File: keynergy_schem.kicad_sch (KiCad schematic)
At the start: 28 parts, among them J1 Conn_01x04_Pin, J2 Conn_01x04_Pin, J3 Conn_01x02_Pin, J4 Conn_01x04_Pin, J5 Conn_01x04_Pin, J6 Conn_01x04_Pin, J8 Conn_01x04_Pin

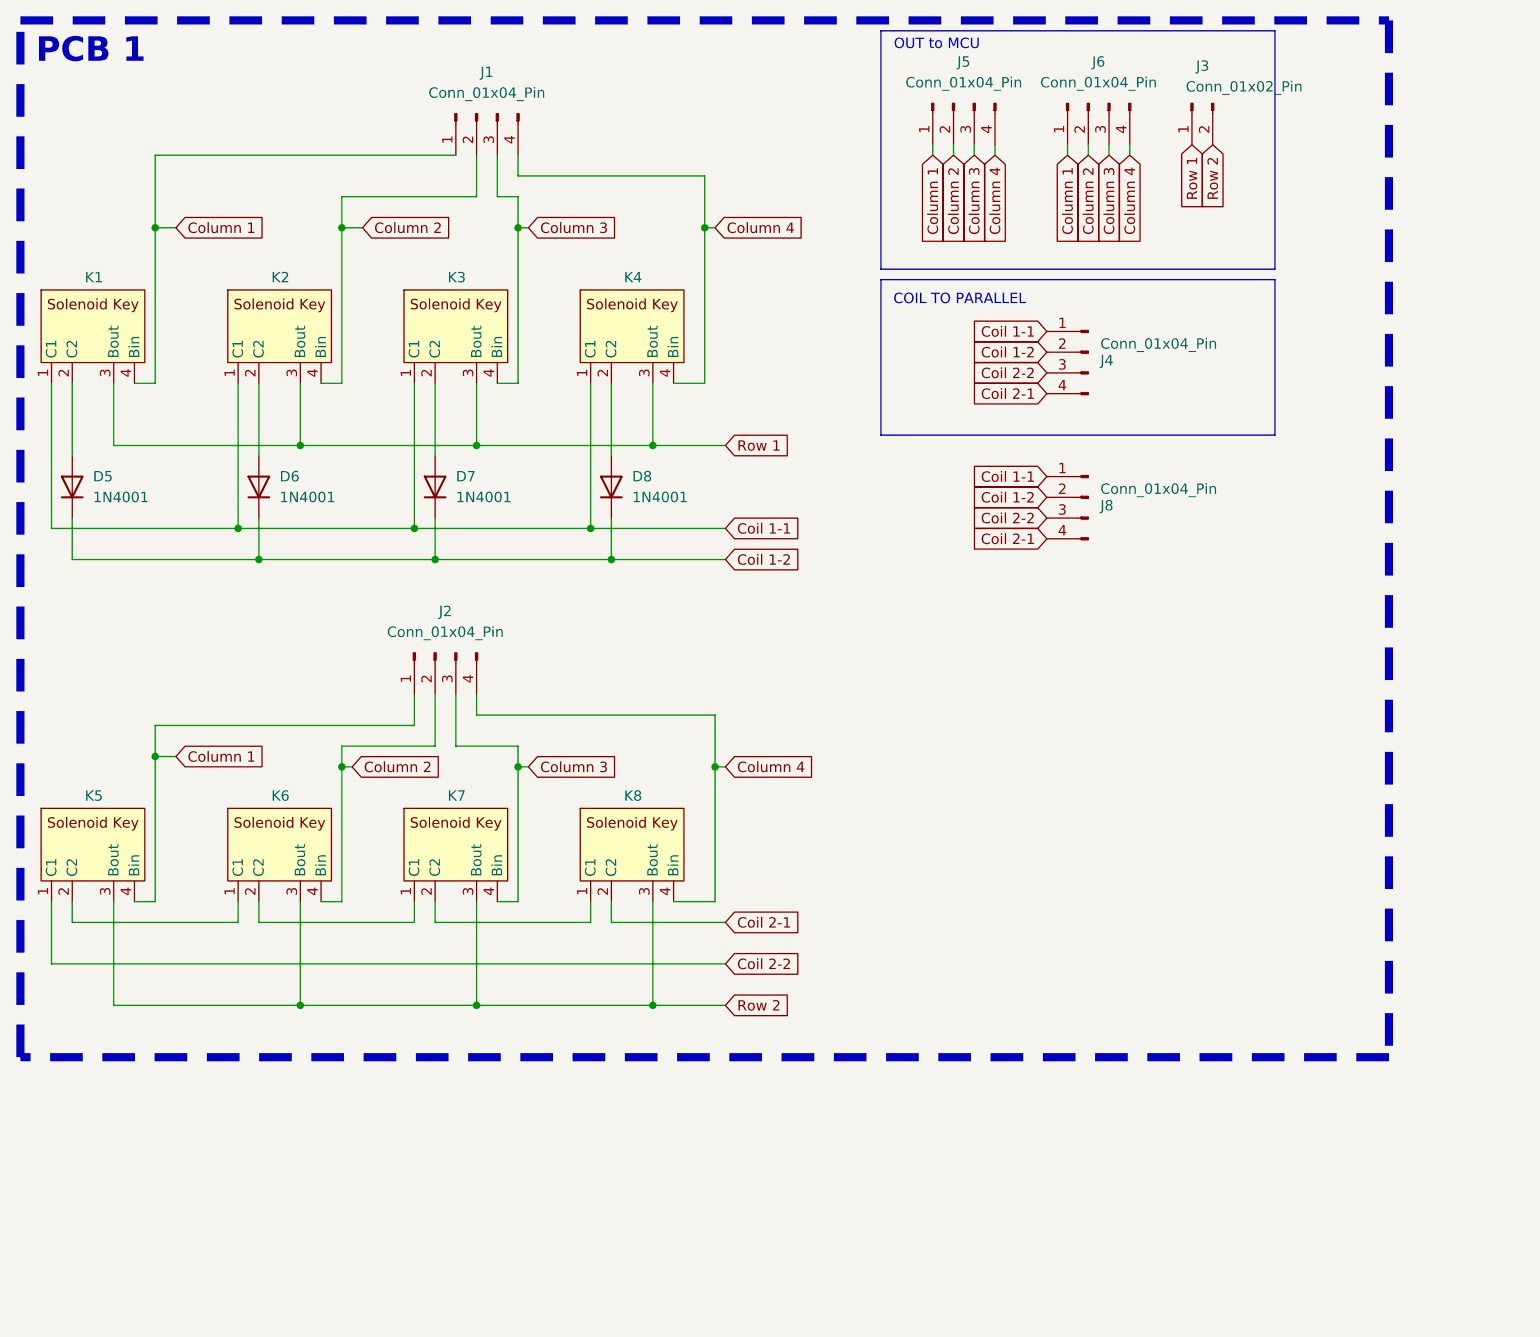
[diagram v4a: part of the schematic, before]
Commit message: new
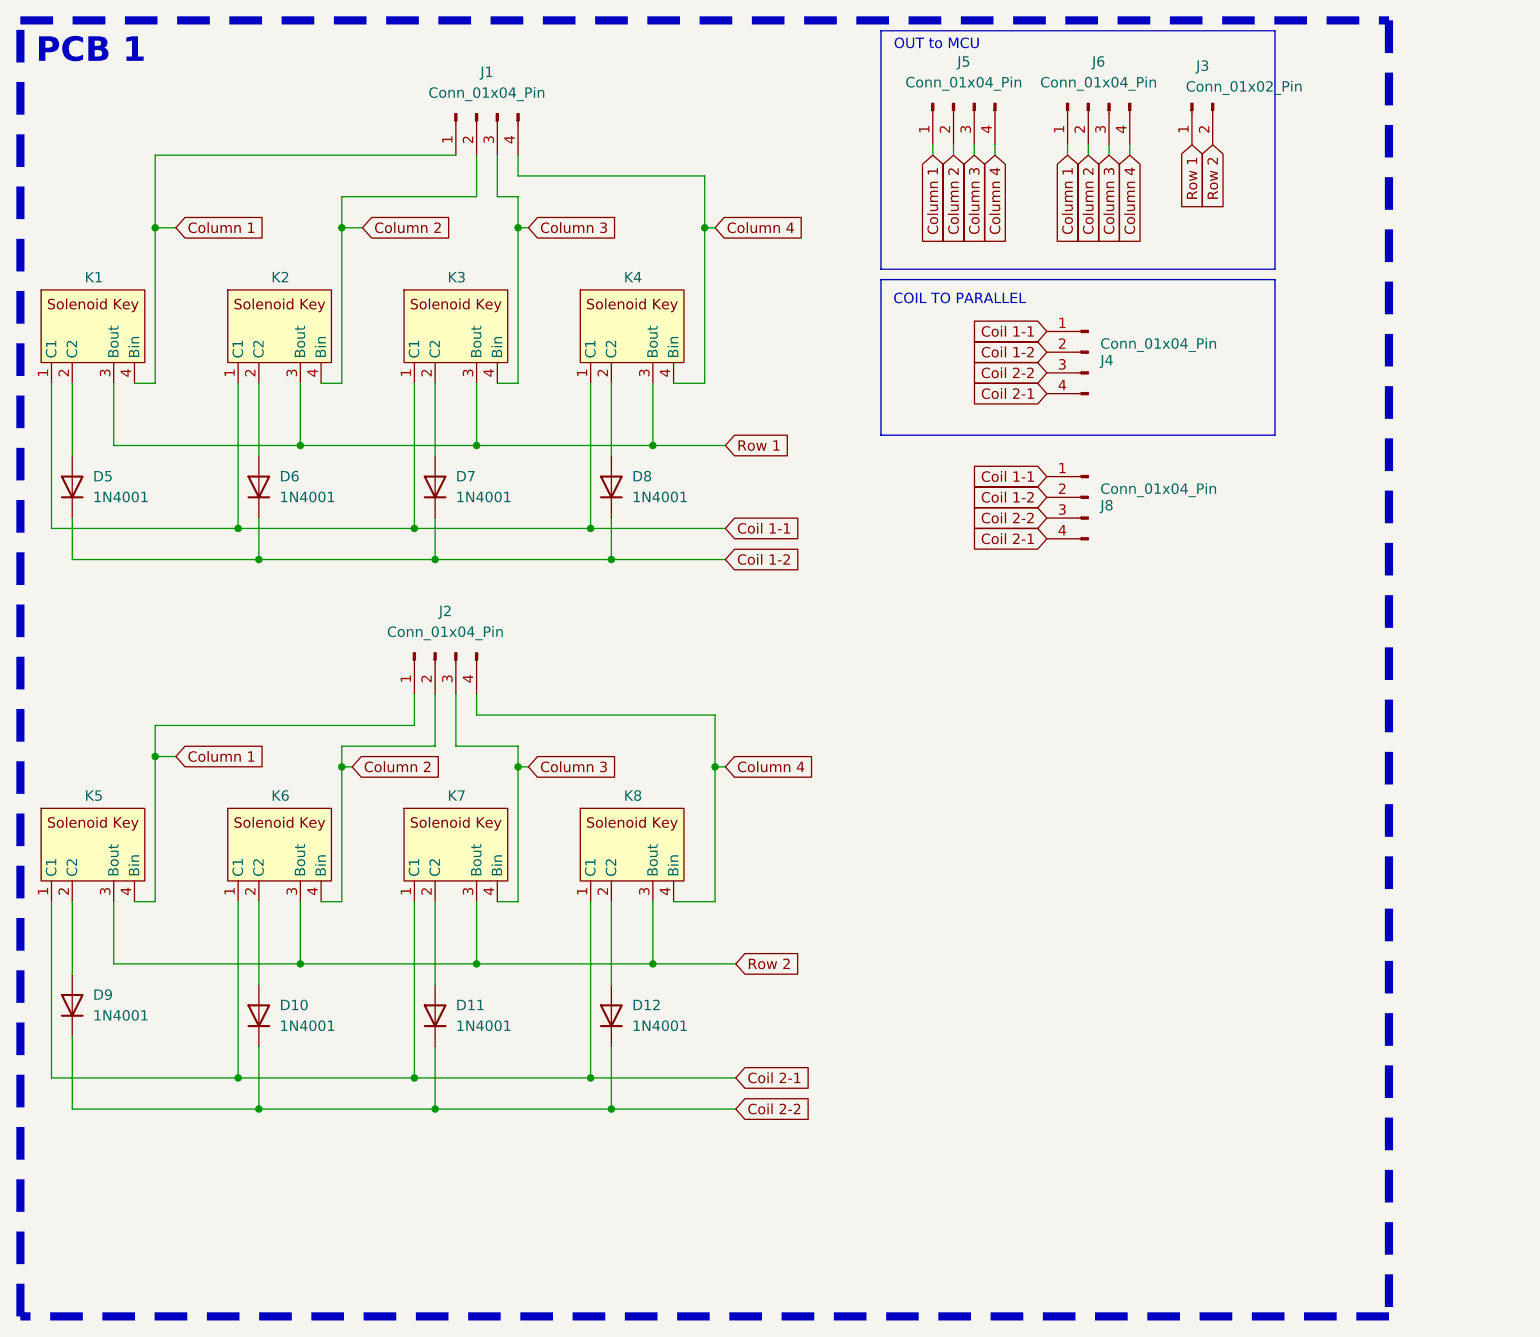
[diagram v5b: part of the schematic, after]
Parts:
- added D10, D11, D12, D9: 1N4001, Diode_THT:D_DO-34_SOD68_P7.62mm_Horizontal, symbol Device:D
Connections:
- net Coil 2-1: now also K5.1 (C1), K6.1 (C1), K7.1 (C1), K8.1 (C1); no longer K8.2 (C2)
- net Coil 2-2: now also D10.1 (K), D11.1 (K), D12.1 (K), D9.1 (K); no longer K5.1 (C1)
- net at K6.2 (C2): now also D10.2 (A); no longer K7.1 (C1)
- net at K7.2 (C2): now also D11.2 (A); no longer K8.1 (C1)
- net at K5.2 (C2): now also D9.2 (A); no longer K6.1 (C1)
- new net: D12.2 (A), K8.2 (C2)

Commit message: new
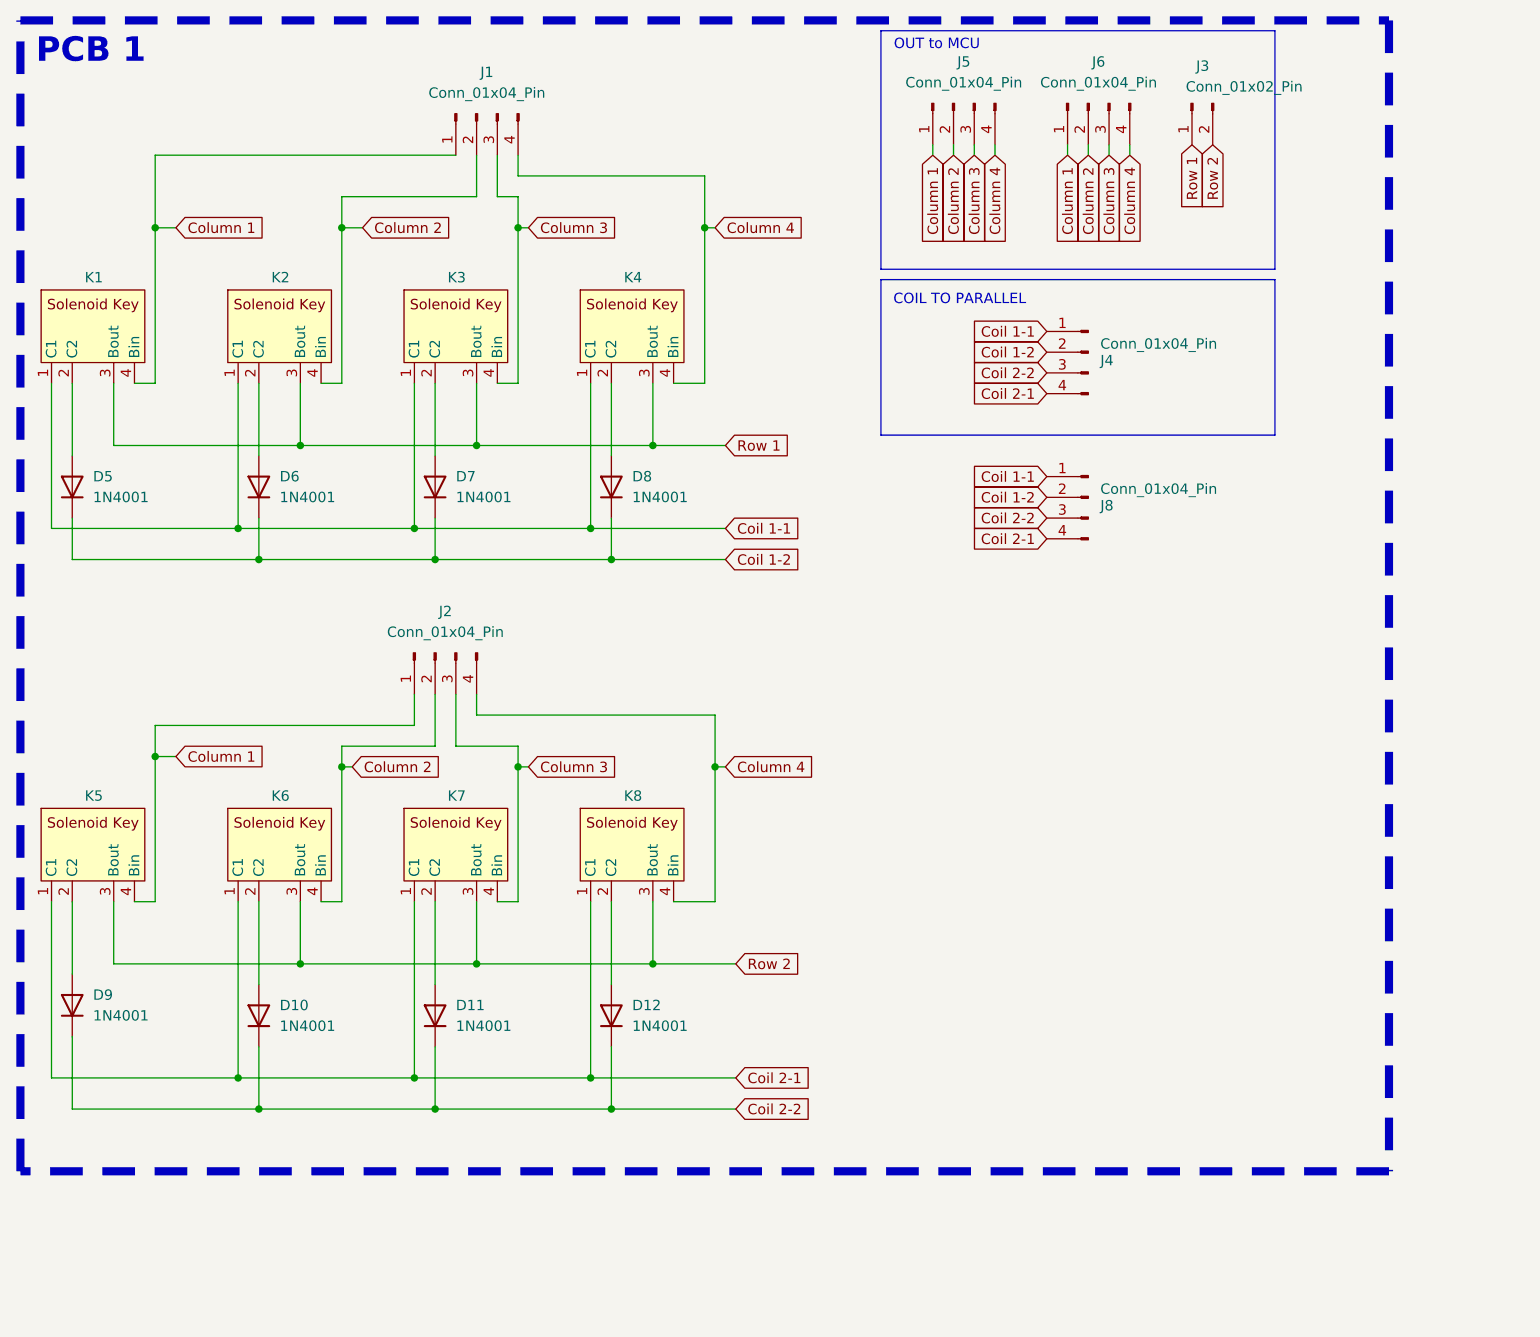
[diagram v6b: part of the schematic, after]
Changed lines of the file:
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@@
 	(rectangle
 		(start 13.97 12.7)
-		(end 181.61 171.45)
+		(end 181.61 153.67)
 		(stroke
 			(width 1)

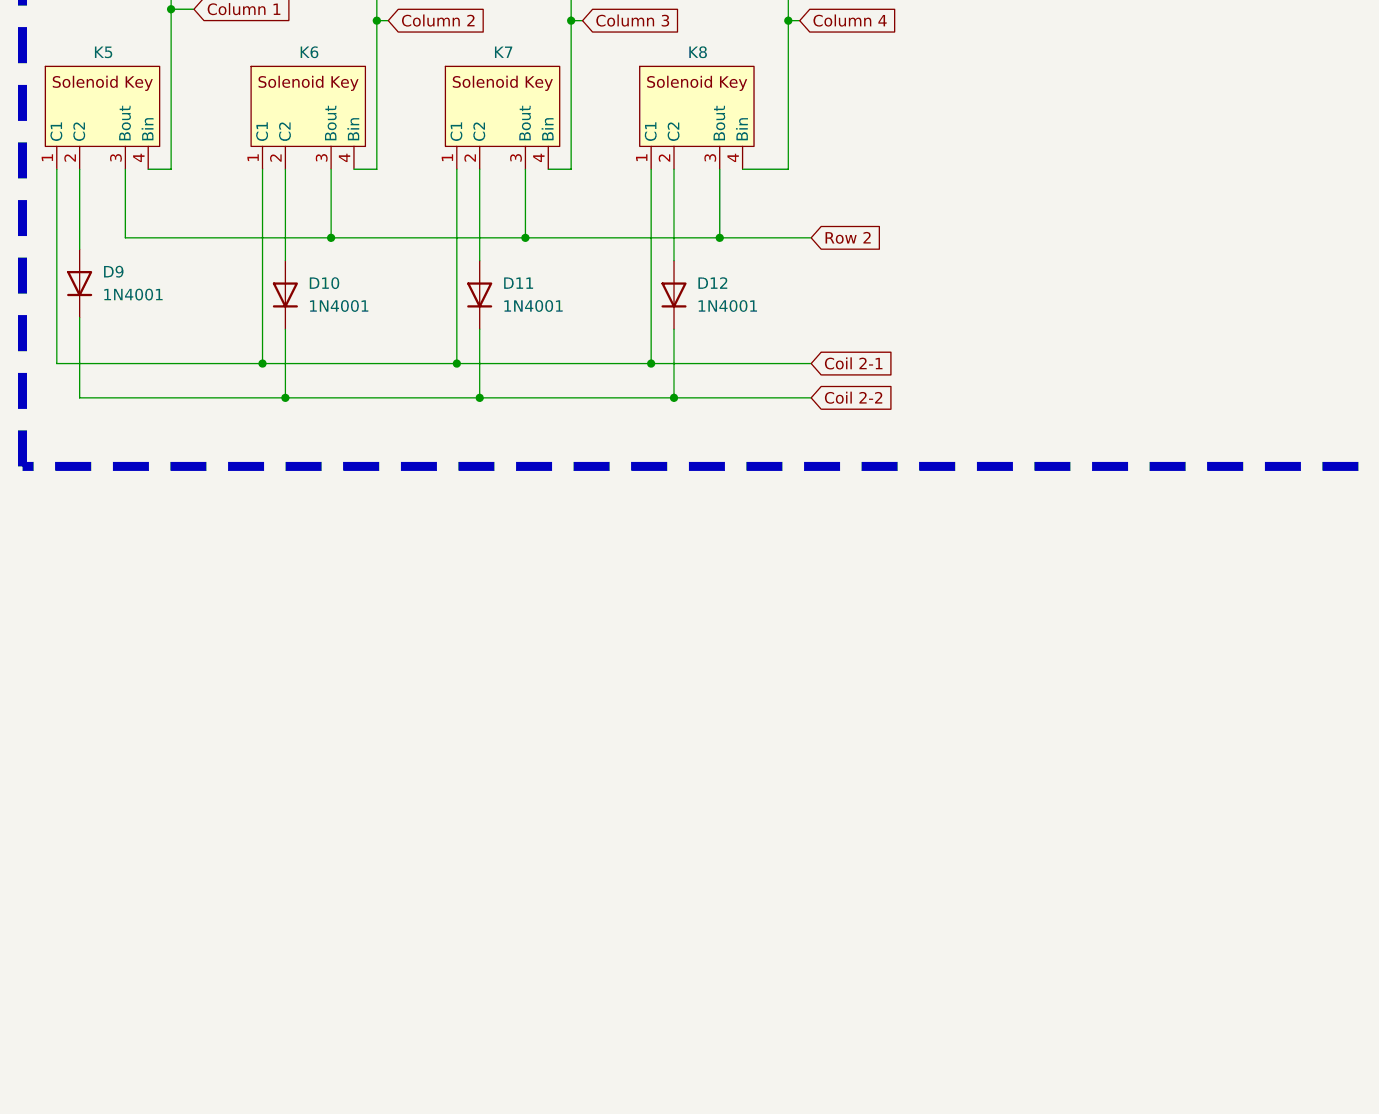
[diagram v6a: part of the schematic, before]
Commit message: new
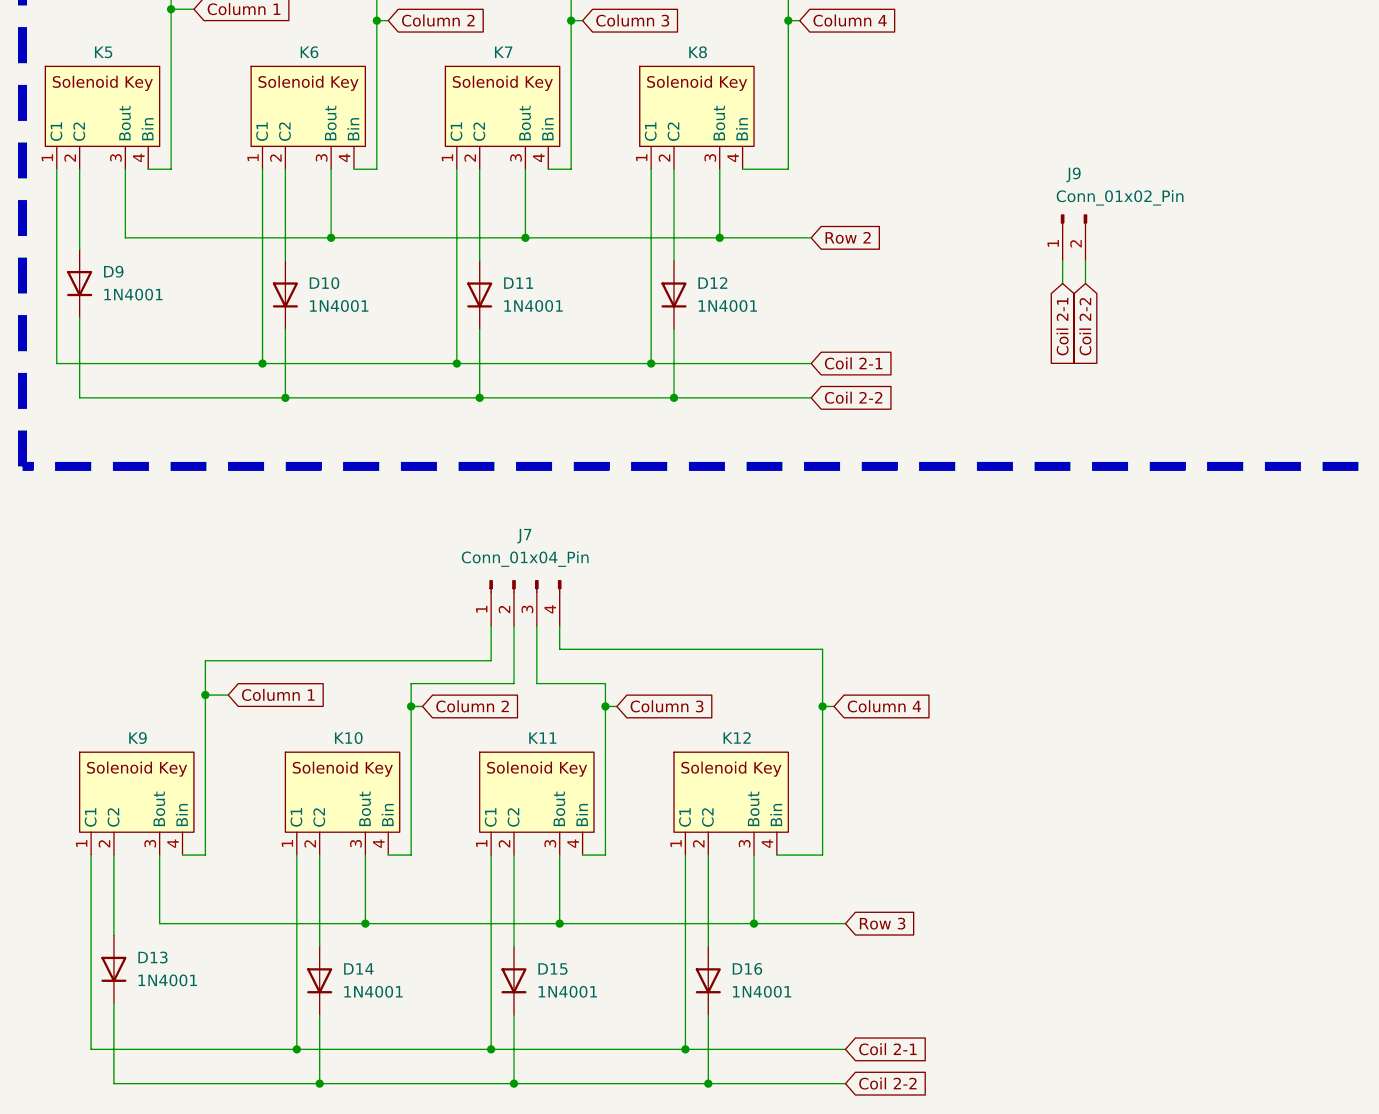
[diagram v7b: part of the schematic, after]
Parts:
- added D13, D14, D15, D16: 1N4001, Diode_THT:D_DO-34_SOD68_P7.62mm_Horizontal, symbol Device:D
- added J7: Conn_01x04_Pin, Connector_PinHeader_2.54mm:PinHeader_1x04_P2.54mm_Vertical, symbol Connector:Conn_01x04_Pin
- added J9: Conn_01x02_Pin, Connector_PinHeader_2.54mm:PinHeader_1x02_P2.54mm_Vertical, symbol Connector:Conn_01x02_Pin
- added K10, K11, K12, K9: ~, project library:Solenoid Key, symbol Key_symbol:Solenoid_Key
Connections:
- net Coil 2-1: now also J9.1 (Pin_1), K10.1 (C1), K11.1 (C1), K12.1 (C1), K9.1 (C1)
- net Coil 2-2: now also D13.1 (K), D14.1 (K), D15.1 (K), D16.1 (K), J9.2 (Pin_2)
- net Column 1: now also J7.1 (Pin_1), K9.4 (Bin)
- net Column 2: now also J7.2 (Pin_2), K10.4 (Bin)
- net Column 3: now also J7.3 (Pin_3), K11.4 (Bin)
- net Column 4: now also J7.4 (Pin_4), K12.4 (Bin)
- new net: D14.2 (A), K10.2 (C2)
- new net: D16.2 (A), K12.2 (C2)
- new net: D13.2 (A), K9.2 (C2)
- new net: D15.2 (A), K11.2 (C2)
- new net Row 3: K10.3 (Bout), K11.3 (Bout), K12.3 (Bout), K9.3 (Bout)
